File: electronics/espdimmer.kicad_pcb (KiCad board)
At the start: 2 copper layers, 86.9 x 18.8 mm, 19 parts, among them J10 LED2, J5 UART, J6 Motion, J7 PWR1, J8 PWR2, J9 LED1, Q1 IRLB3034, Q2 IRLB3034, SW1 Reset, SW2 Flash, U1 ESP-01v090

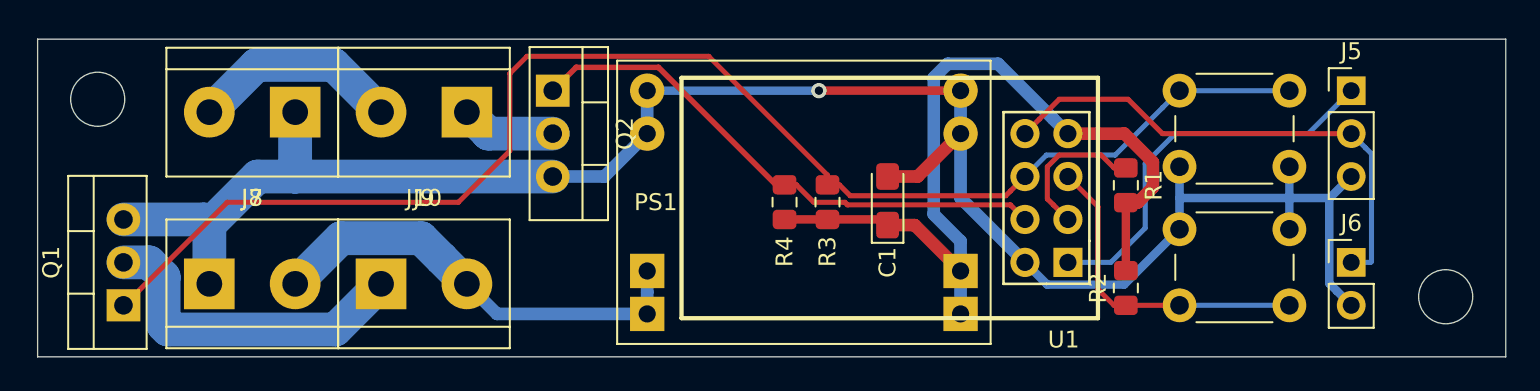
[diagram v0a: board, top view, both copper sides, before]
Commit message: Schematics and PCB design updated
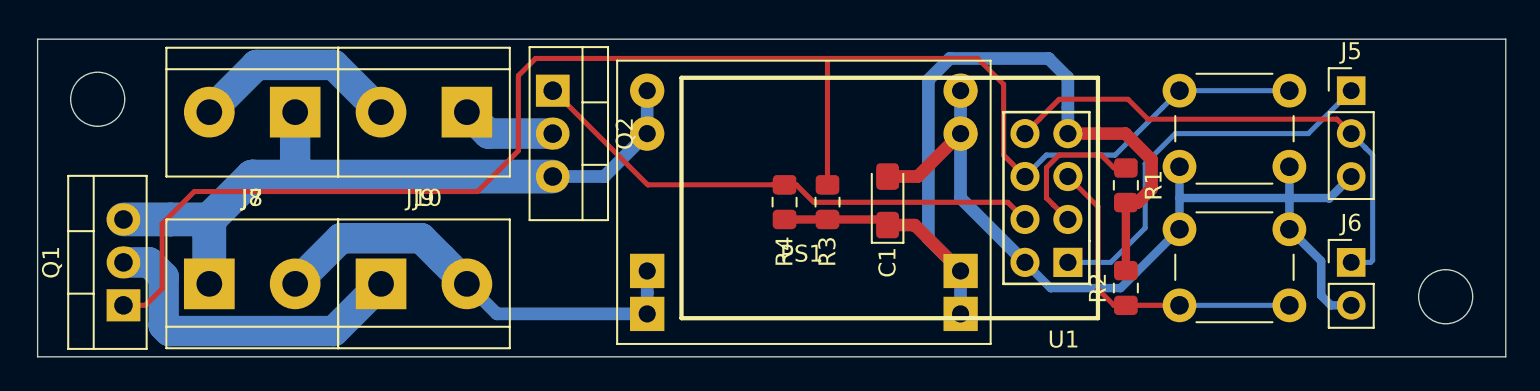
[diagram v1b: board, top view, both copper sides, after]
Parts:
- PS1: value BUCK -> BUCK_4P; footprint ESPDimmer:XM1584_buck_module -> Buck:XM1584_buck_mod_4p
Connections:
- net Net-(J10-Pad2) renamed /PWR2
- net Net-(J7-Pad2) renamed /PWR1
- J7 pad 1: GND -> GNDD
- J8 pad 1: GND -> GNDD
- PS1 pad 1: GND -> GNDD
- PS1 pad 3: +3V3 -> GND
- Q1 pad 3: GND -> GNDD
- Q2 pad 3: GND -> GNDD
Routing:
- net GND: track 114.9 -> 53.2 mm, vias 1 -> 0
- net GNDD: track 0.00 -> 43.3 mm
- net Net-(Q1-Pad1): track 84.1 -> 94.8 mm
- net +3V3: track 49.5 -> 52.1 mm
- net Net-(Q2-Pad1): track 32.2 -> 31.1 mm
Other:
- net class Default: clearance 0.2 -> 0.25
- net class PWR: clearance 0.2 -> 0.25; trace_width 2 -> 1.8
- net class VCC: clearance 0.2 -> 0.25
- rule trace_clearance: 0.2 -> 0.25
